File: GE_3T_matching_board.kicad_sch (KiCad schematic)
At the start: 10 parts

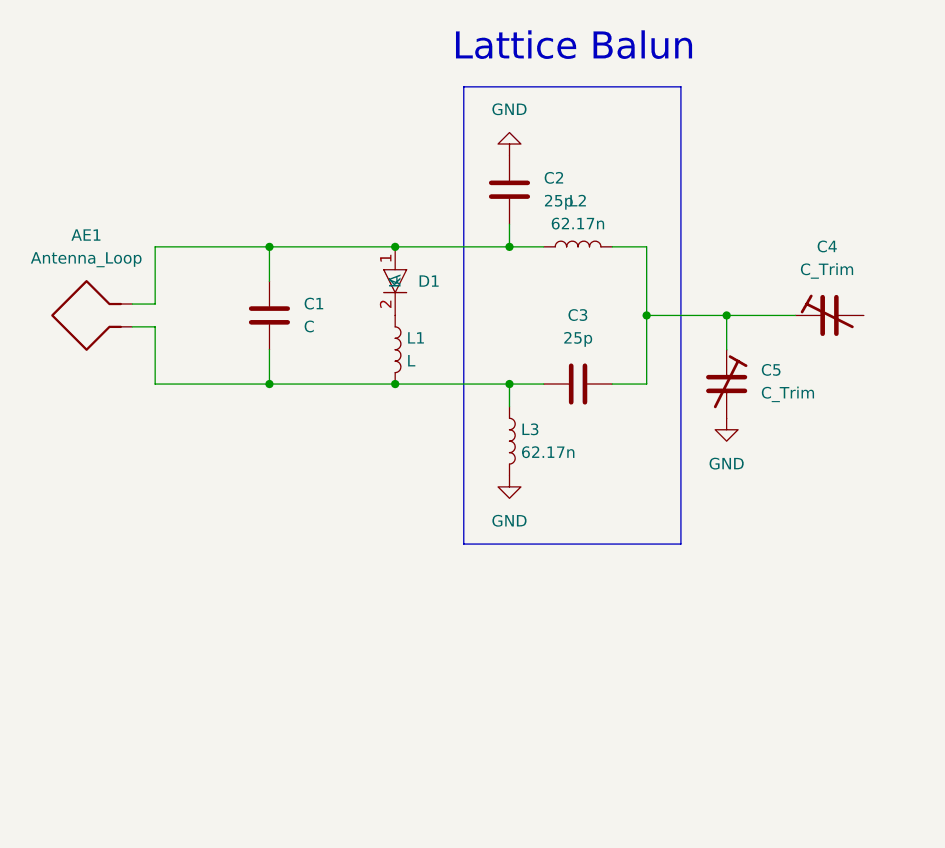
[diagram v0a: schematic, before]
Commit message: send to Nibardo to check
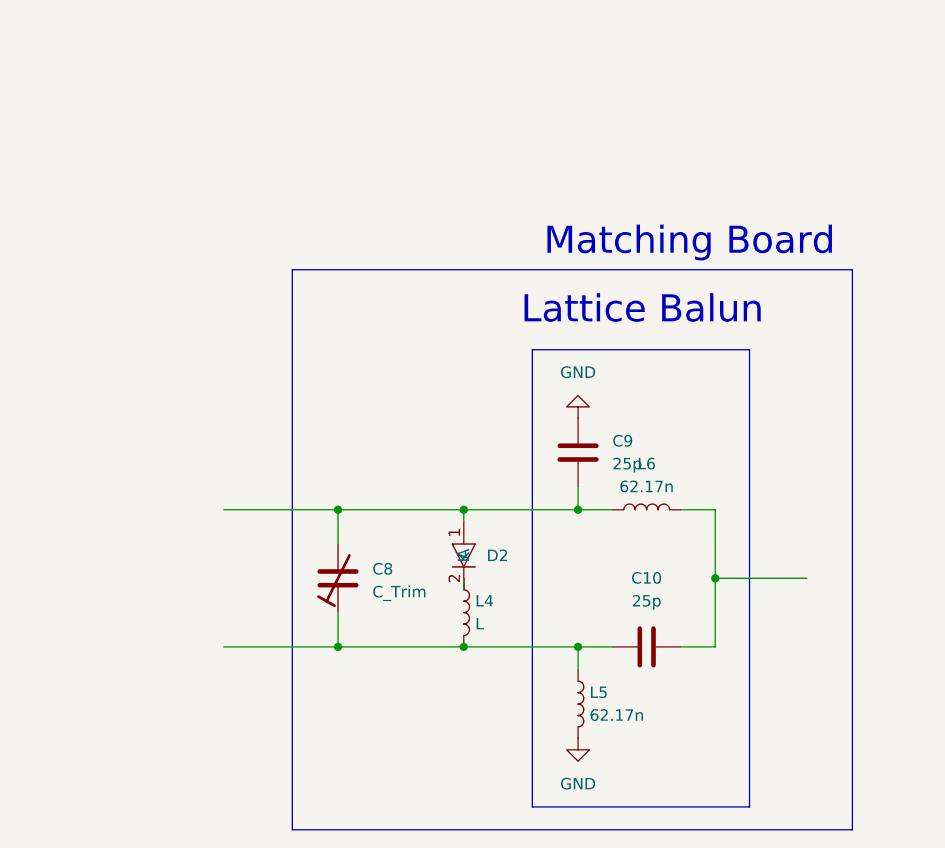
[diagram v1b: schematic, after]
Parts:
- removed AE1: Antenna_Loop, symbol Device:Antenna_Loop
- removed C1: C, aaa_MyLib:CAP_1111_HIQ_KNO, symbol Device:C
- removed C2, C3: 25p, aaa_MyLib:CAP_1111_HIQ_KNO, symbol Device:C
- removed C4, C5: C_Trim, symbol Device:C_Trim
- removed D1: ~, aaa_MyLib:PIN_diode_NonMagnetic_HighPower, symbol AAA_MyLib:PinDiode_NonMagnetic_HighPower
- removed L1: L, symbol Device:L
- removed L2: 62.17n, aaa_MyLib:CAP_1111_HIQ_KNO, symbol Device:L
- removed L3: 62.17n, symbol Device:L
- added C10, C9: 25p, aaa_MyLib:CAP_1111_HIQ_KNO, symbol Device:C
- added C8: C_Trim, aaa_MyLib:CAP_1111_HIQ_KNO, symbol Device:C_Trim
- added D2: ~, aaa_MyLib:PIN_diode_NonMagnetic_HighPower, symbol AAA_MyLib:PinDiode_NonMagnetic_HighPower
- added L4: L, aaa_MyLib:CAP_1111_HIQ_KNO, symbol Device:L
- added L5, L6: 62.17n, aaa_MyLib:CAP_1111_HIQ_KNO, symbol Device:L
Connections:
- net GND: now also C9.1, L5.2
- new net: C8.2, C9.2, D2.1 (A), L6.1
- new net: D2.2 (K), L4.1
- new net: C10.1, C8.1, L4.2, L5.1
- new net: C10.2, L6.2
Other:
- note added: "Matching Board"
